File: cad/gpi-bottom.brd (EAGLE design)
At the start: 130 x 73.5 mm, 4 parts, among them CN1 HEADER-3X12MM

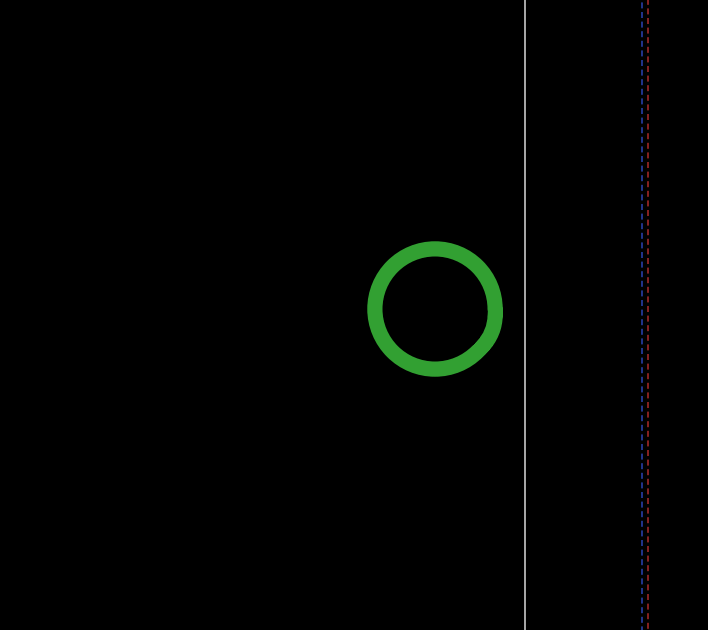
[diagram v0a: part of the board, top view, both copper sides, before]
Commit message: caps
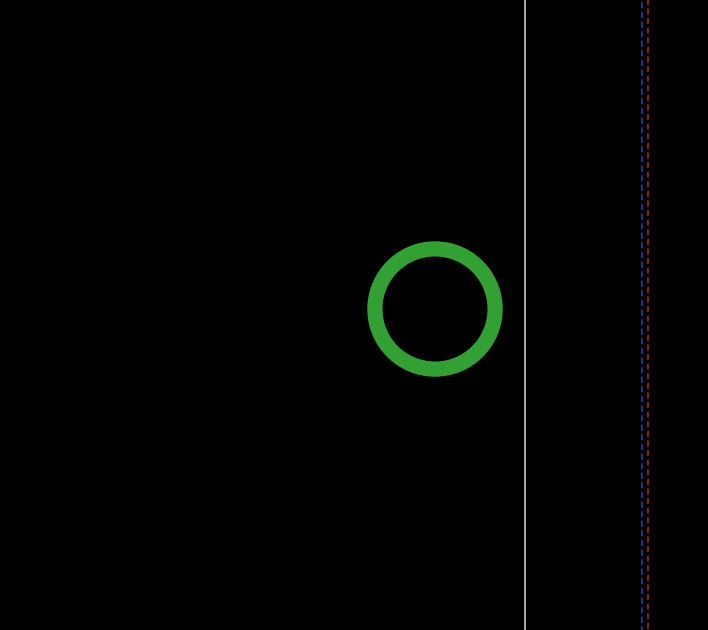
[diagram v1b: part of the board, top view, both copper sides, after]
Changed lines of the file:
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@@
 </class>
 </classes>
-<designrules name="default">
+<designrules name="default *">
 <description language="de">&lt;b&gt;EAGLE Design Rules&lt;/b&gt;
 &lt;p&gt;
@@
 <param name="mdViaViaSameLayer" value="8mil"/>
 <param name="mnLayersViaInSmd" value="2"/>
-<param name="mdCopperDimension" value="40mil"/>
+<param name="mdCopperDimension" value="1mil"/>
 <param name="mdDrill" value="8mil"/>
 <param name="mdSmdStop" value="0mil"/>
-<param name="msWidth" value="10mil"/>
+<param name="msWidth" value="0.25mm"/>
 <param name="msDrill" value="24mil"/>
 <param name="msMicroVia" value="9.99mm"/>
@@
 <via x="109.5" y="8.8" extent="1-16" drill="2.5"/>
 <via x="118" y="73" extent="1-16" drill="2"/>
-<via x="127.5" y="15.8" extent="1-16" drill="2.5"/>
 <via x="21.5" y="12.3" extent="1-16" drill="2.5"/>
 <via x="21.5" y="15.8" extent="1-16" drill="2.5"/>
